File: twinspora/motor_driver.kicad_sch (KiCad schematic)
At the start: 18 parts, among them J14 Conn_01x03, U6 DRV8316CRRGFR

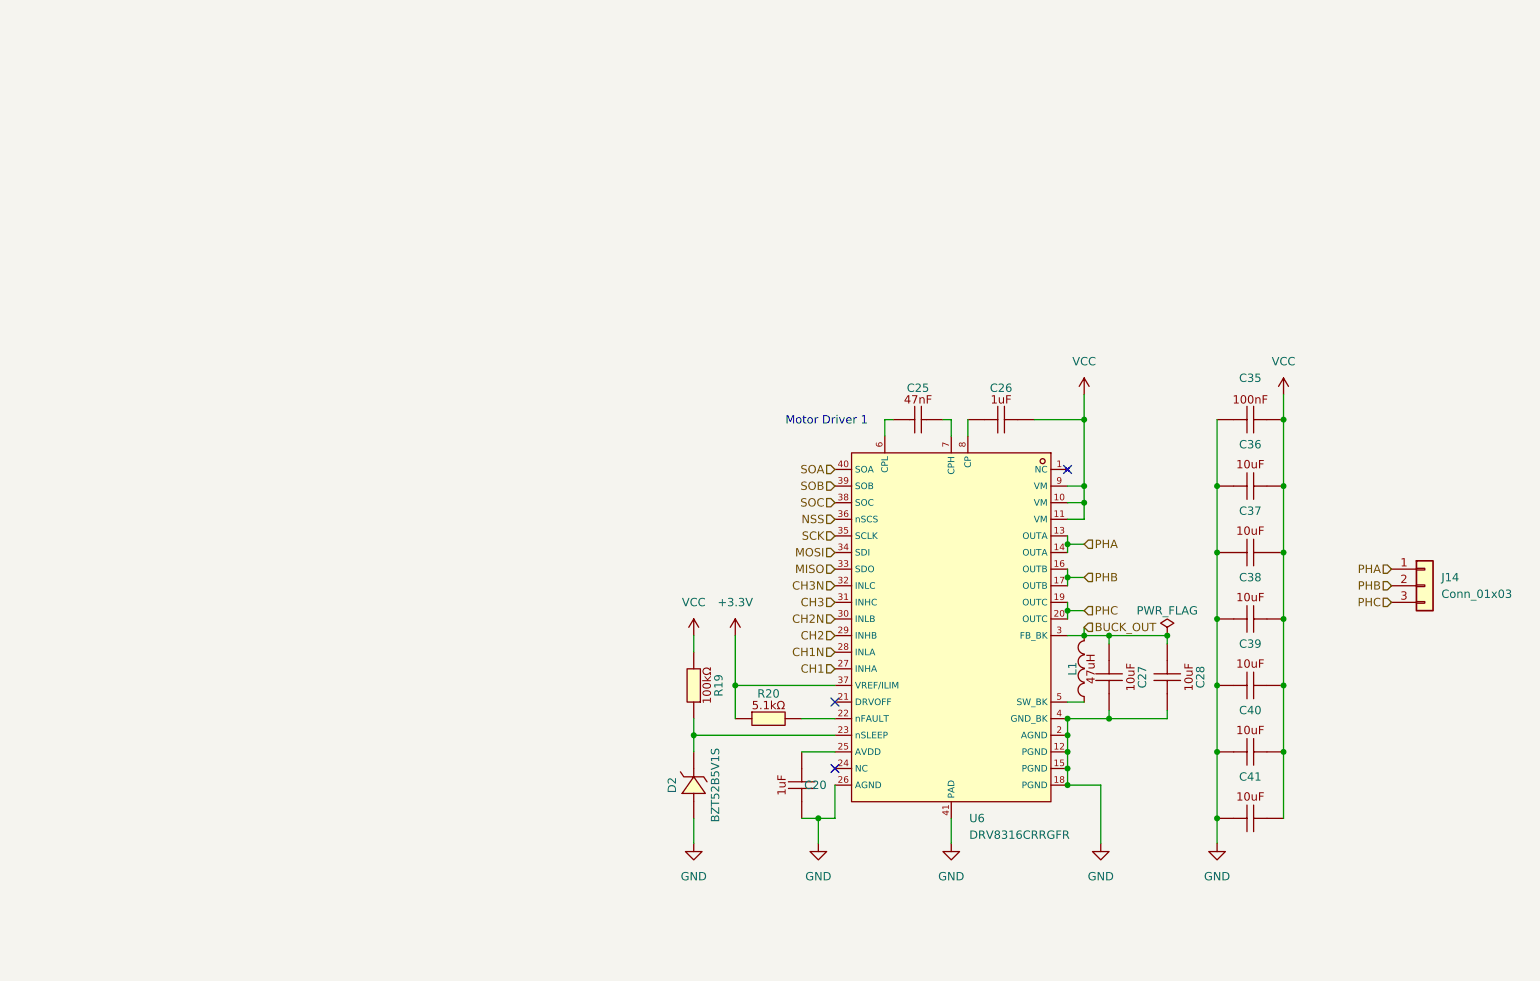
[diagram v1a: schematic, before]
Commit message: NEW
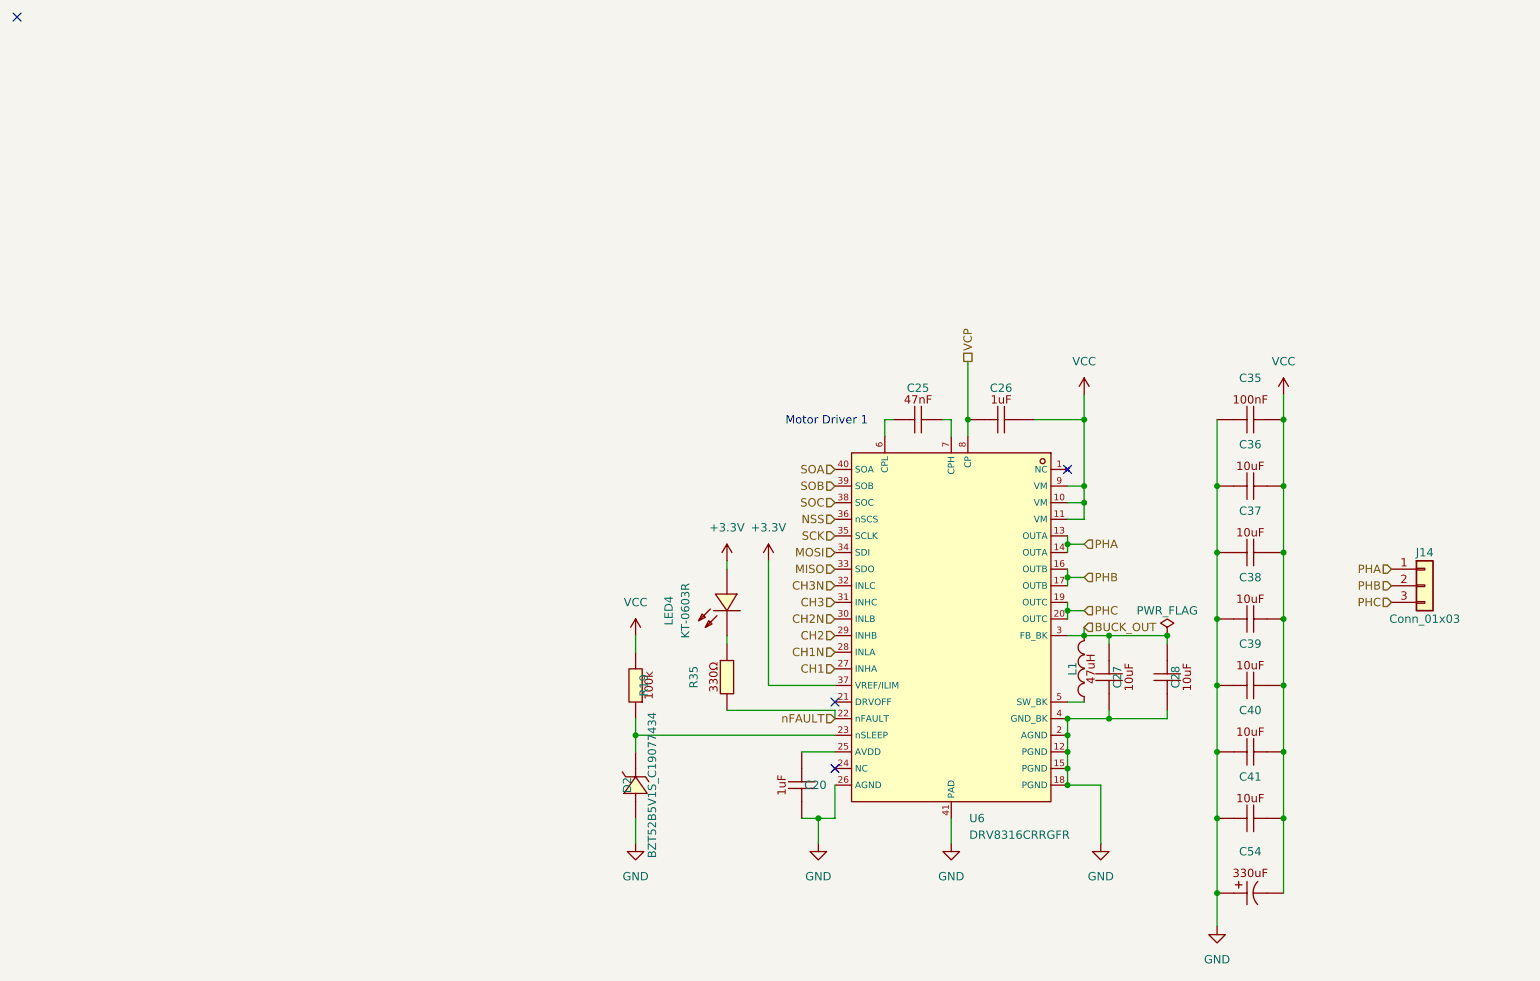
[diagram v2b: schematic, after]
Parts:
- removed R20: 0402WGF5101TCE, Basic_Capacitors_Resistors:R0402, symbol Basic_Capacitors_Resistors:0402WGF5101TCE
- added C54: EEEFT1H331GP, Capacitor_SMD_UWRL:CAP-SMD_BD10.0-L10.3-W10.3-LS11.0-R-RD, symbol Capacitor_SMD_UWRL:EEEFT1H331GP
- added LED4: KT-0603R, LED:LED0603-RD, symbol LED:KT-0603R
- added R35: 0402WGF3300TCE, Resistor_SMD:R_0402_1005Metric, symbol Basic_Capacitors_Resistors:0402WGF3300TCE
- C27, C28, C36, C37, C38, C39, C40, C41: footprint Basic_Capacitors_Resistors:C0805 -> Capacitor_SMD:C_0805_2012Metric
- C35: footprint Basic_Capacitors_Resistors:C0402 -> Capacitor_SMD:C_0402_1005Metric
- D2: value BZT52B5V1S -> BZT52B5V1S_C19077434; footprint Diode:SOD-323_L1.7-W1.3-LS2.6-RD -> Diode_SMD:D_SOD-323_HandSoldering
- J14: footprint Connector_DORABO:CONN-TH_DB125-2.54-3P-GN -> (none)
- R19: footprint Basic_Capacitors_Resistors:R0402 -> Resistor_SMD:R_0402_1005Metric
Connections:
- net +3.3V: now also LED4.2 (A)
- net GND: now also C54.1
- net VCC: now also C54.2
- net VCP: now reaches C26.2, U6.8 (CP)
- net nFAULT: now reaches U6.22 (nFAULT)
- net nFAULT: now also R35.2
- new net: LED4.1 (K), R35.1
- no-connect marks 3 -> 4
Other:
- moved on the sheet: D2, R19
